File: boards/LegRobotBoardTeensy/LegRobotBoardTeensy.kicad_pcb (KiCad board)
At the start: 2 copper layers, 109.6 x 116.6 mm, 116 parts, among them J1 IDC, J10 IDC, J11 IDC, J12 IDC, J13 IDC, J14 IDC, J15 IDC, J16 IDC, J2 B3B-XH-A, J3 B3B-XH-A, J4 B3B-XH-A, J5 B3B-XH-A, J6 IDC, J7 IDC, J8 IDC, J9 IDC, Q1 MMBT3904LT1G, Q10 MMBT3904LT1G, Q11 MMBT3904LT1G, Q12 MMBT3904LT1G, Q13 MMBT3904LT1G, Q14 MMBT3904LT1G, Q15 MMBT3904LT1G, Q16 MMBT3904LT1G, Q17 MMBT3904LT1G, Q18 MMBT3904LT1G, Q19 MMBT3904LT1G, Q2 MMBT3904LT1G, Q20 MMBT3904LT1G, Q21 MMBT3904LT1G, Q22 MMBT3904LT1G, Q23 MMBT3904LT1G, Q24 MMBT3904LT1G, Q3 MMBT3904LT1G, Q4 MMBT3904LT1G, Q5 MMBT3904LT1G, Q6 MMBT3904LT1G, Q7 MMBT3904LT1G, Q8 MMBT3904LT1G, Q9 MMBT3904LT1G, U1 Teensy4.0, U2 TLC555CDR, U3 SN74HC08DR, U4 SN74HC08DR, U5 PCA9685PW_118, U6 SN74HC08DR, U7 SN74HC08DR, U8 BNO055

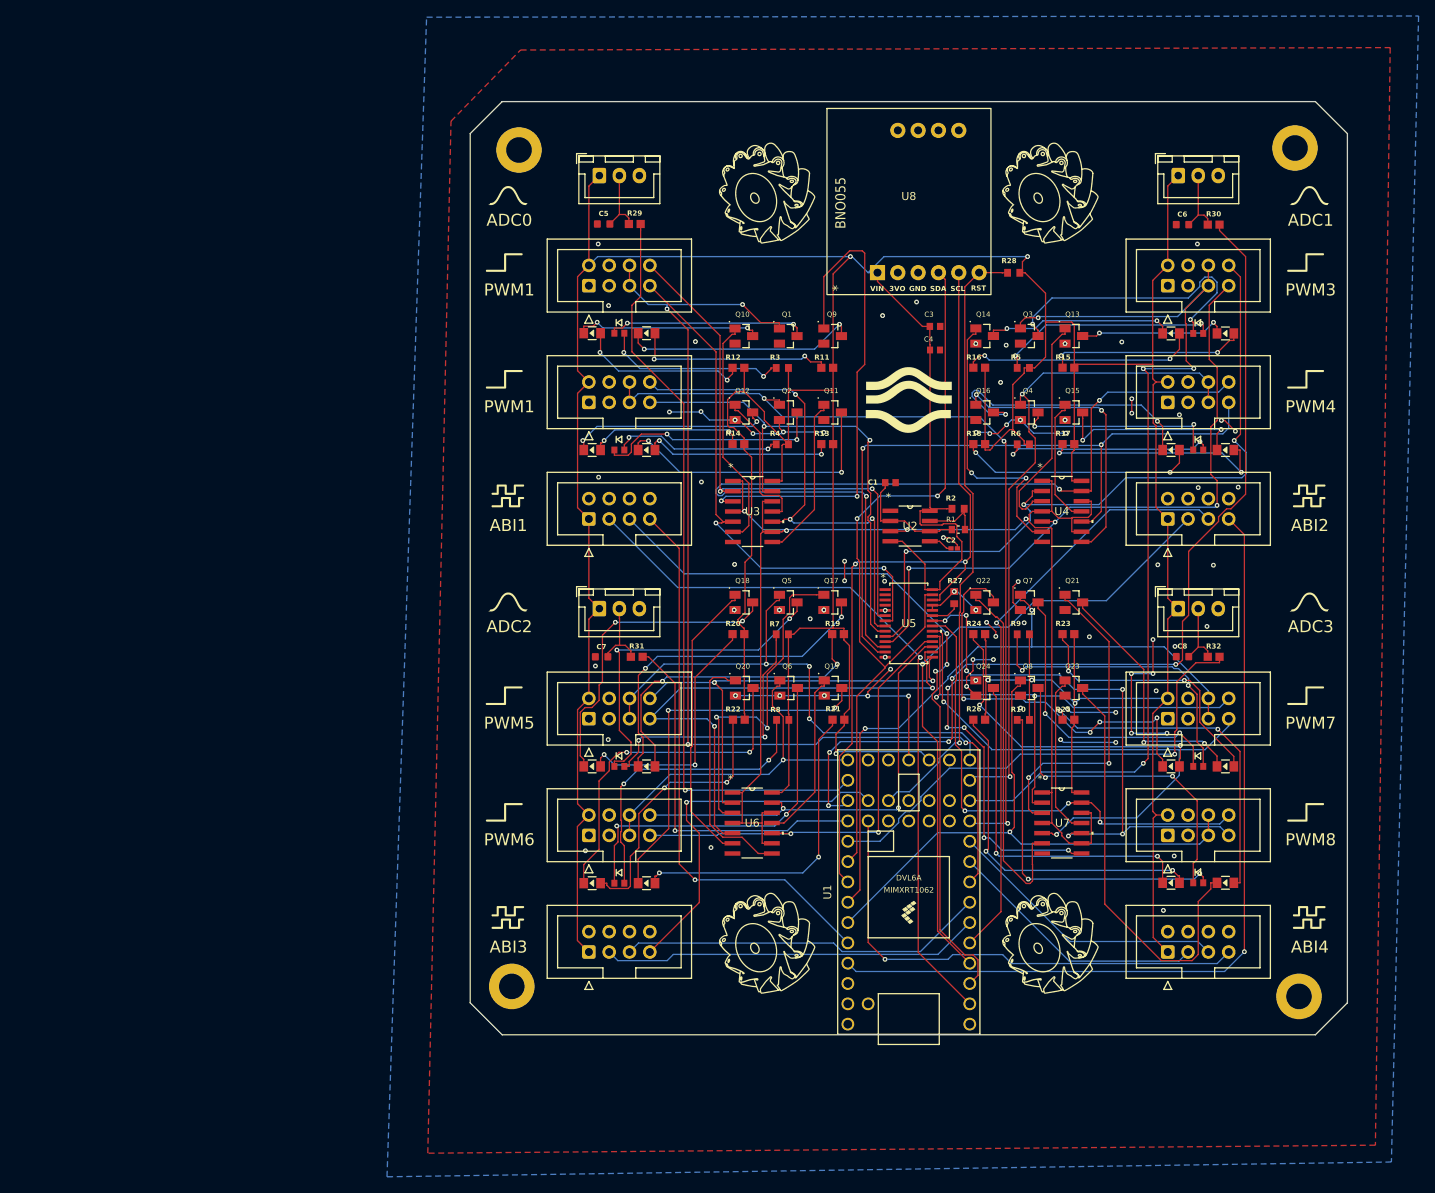
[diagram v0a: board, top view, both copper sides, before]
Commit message: Clean up and document boards
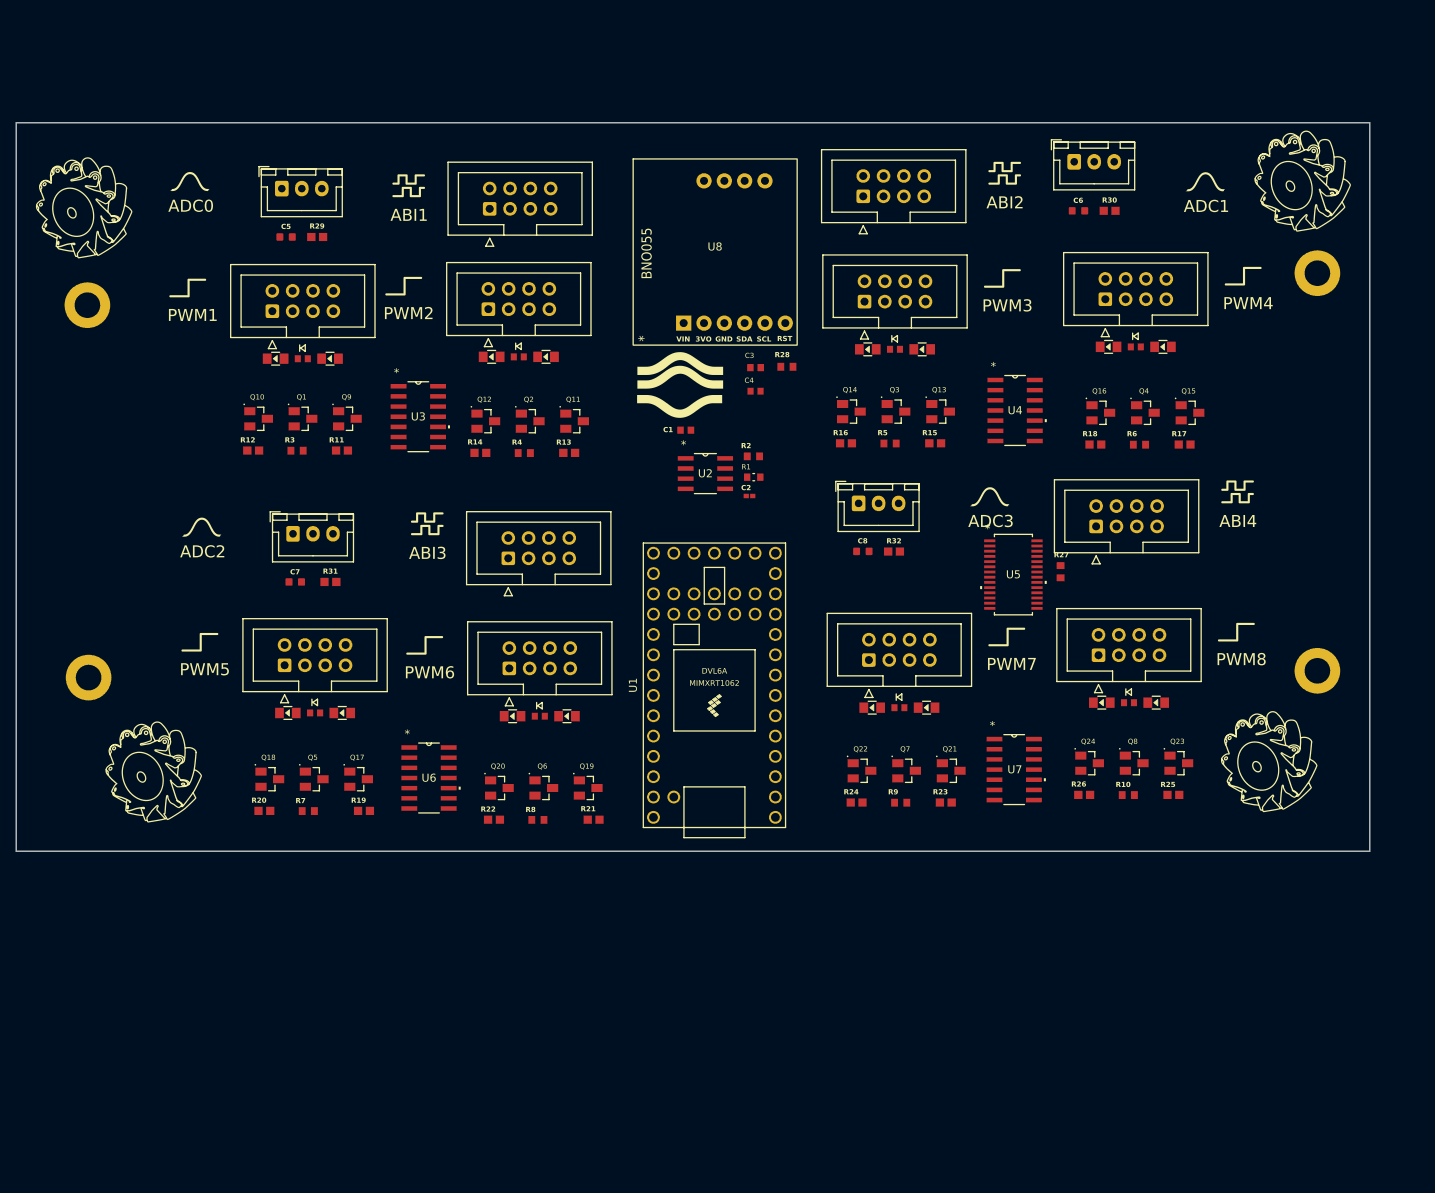
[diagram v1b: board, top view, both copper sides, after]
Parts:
- moved MH3 65.5 mm to (45.6, 102.2)
- moved Q5 63.2 mm to (73.8, 114.9)
- moved Q17 63.2 mm to (79.3, 114.9)
- moved Q18 63.2 mm to (68.2, 114.9)
- moved R20 63.2 mm to (67.6, 118.9)
- moved R7 63.2 mm to (73.1, 118.9)
- moved R19 63.2 mm to (80.0, 118.9)
- moved Q1 61.5 mm to (72.4, 69.8)
- moved Q10 61.5 mm to (66.8, 69.8)
- moved R12 61.5 mm to (66.2, 73.8)
- moved Q9 61.5 mm to (78.0, 69.8)
- moved R11 61.5 mm to (77.3, 73.8)
- moved R3 61.5 mm to (71.7, 73.8)
- moved MH1 57.3 mm to (45.5, 55.6)
- moved J14 55.5 mm to (142.4, 42.0)
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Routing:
- net +3.3V: track 659.3 -> 0.00 mm, vias 6 -> 0
- net BLINK: track 176.5 -> 0.00 mm, vias 4 -> 0
- net PWMEN1: track 134.3 -> 0.00 mm, vias 4 -> 0
- net GND: track 133.7 -> 0.00 mm, vias 79 -> 0
- net A1: track 122.0 -> 0.00 mm, vias 5 -> 0
- net PWMEN3: track 120.4 -> 0.00 mm, vias 4 -> 0
- net RPWM4: track 116.6 -> 0.00 mm, vias 3 -> 0
- net PWMEN2: track 107.7 -> 0.00 mm, vias 3 -> 0
- net ENCODER2_I: track 105.9 -> 0.00 mm, vias 1 -> 0
- net SCL: track 98.9 -> 0.00 mm, vias 2 -> 0
- net SDA: track 98.2 -> 0.00 mm, vias 2 -> 0
- net A0: track 94.8 -> 0.00 mm, vias 1 -> 0
- net ENCODER1_B: track 94.4 -> 0.00 mm, vias 3 -> 0
- net ENCODER1_A: track 92.1 -> 0.00 mm, vias 1 -> 0
- net RPWM3: track 92.0 -> 0.00 mm, vias 3 -> 0
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- removed copper zone on B.Cu, net GND
- removed copper zone on F.Cu, net GND
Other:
- board size 109.6 x 116.6 mm -> 169.2 x 91.1 mm
- board text added: "PWM2"
